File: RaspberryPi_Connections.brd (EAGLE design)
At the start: 124.4 x 101.3 mm, 4 parts

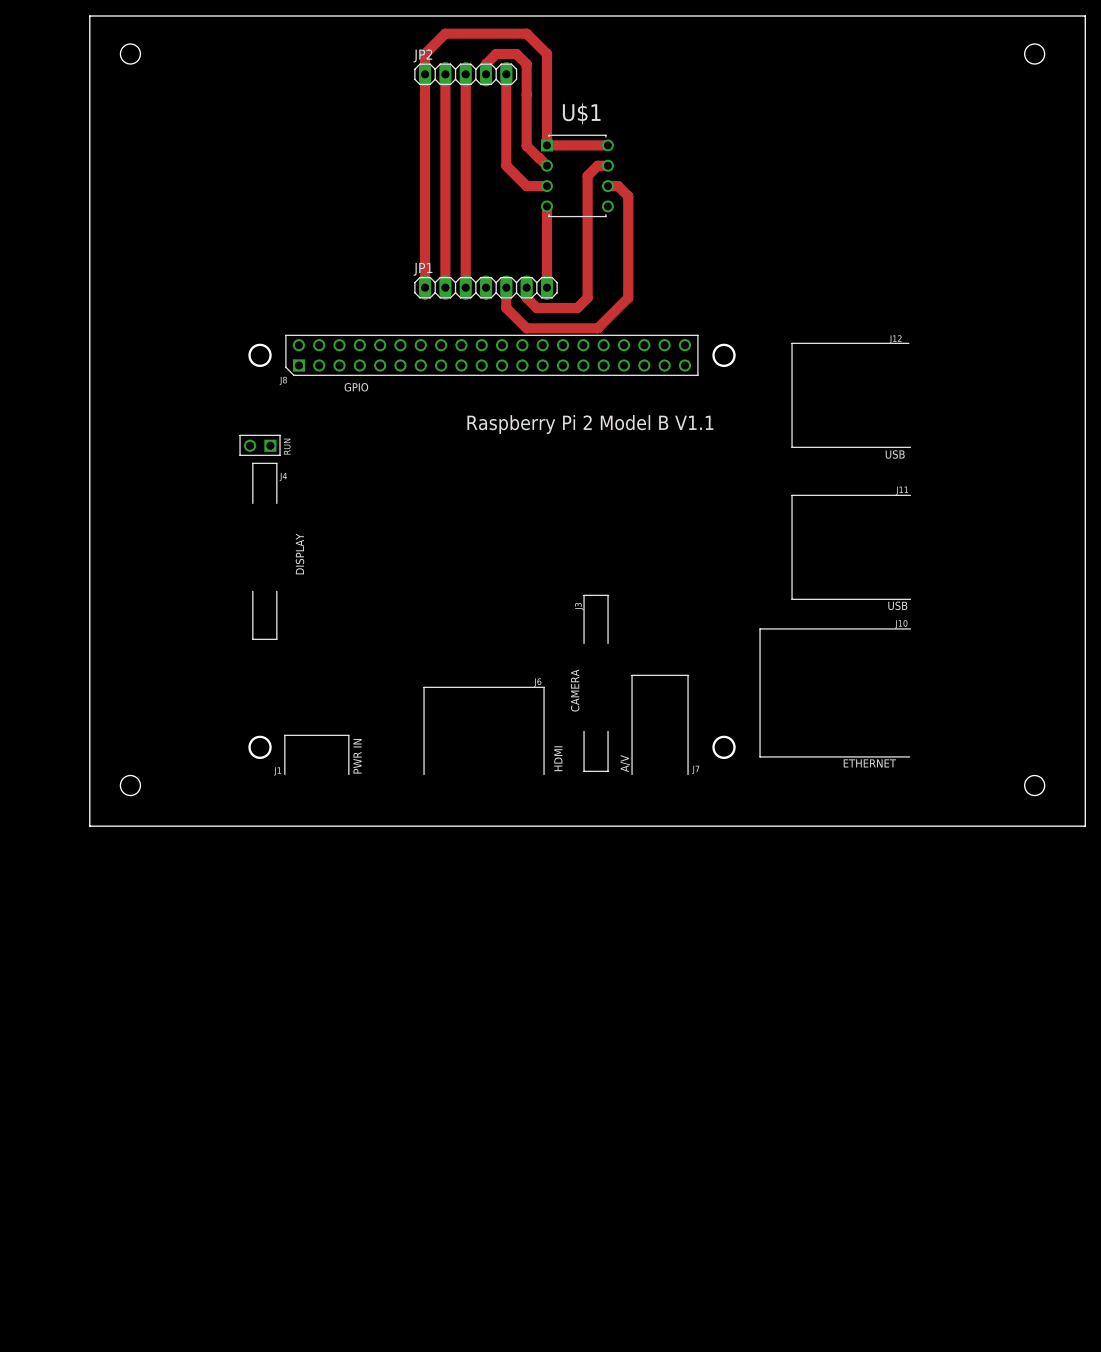
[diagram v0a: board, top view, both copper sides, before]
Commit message: Final update before printing first prototype
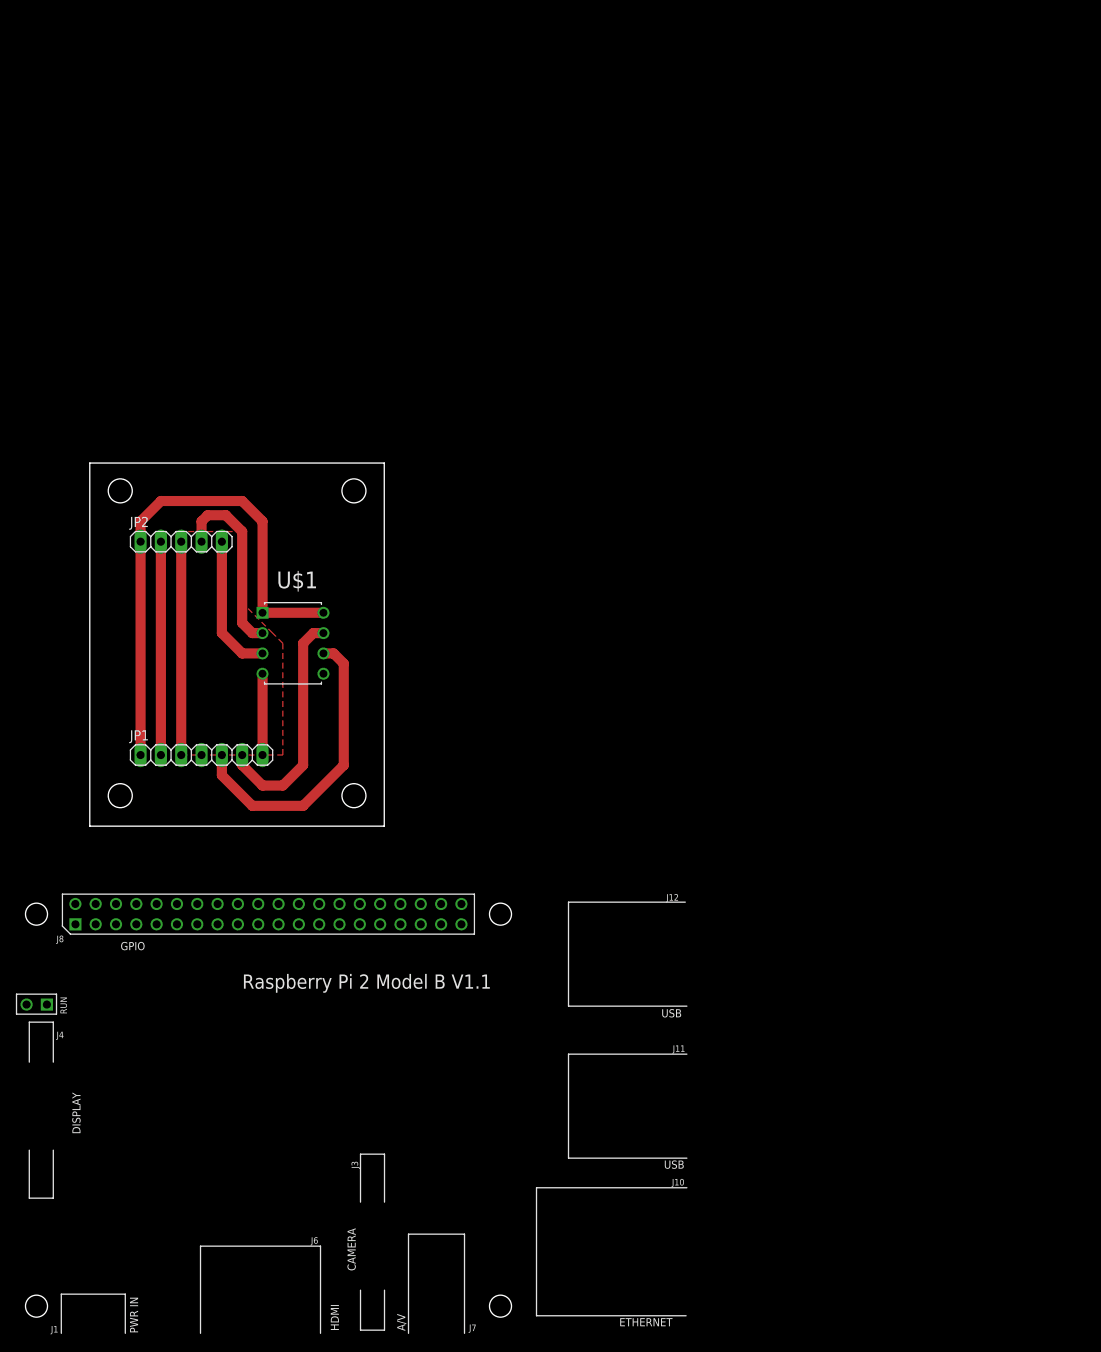
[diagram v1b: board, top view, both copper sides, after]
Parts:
- moved PCB1 75.2 mm to (-10.2, -63.5)
- moved JP1 68.4 mm to (14.0, 8.89)
- moved JP2 68.4 mm to (11.4, 35.6)
- moved U$1 68.4 mm to (29.2, 19.1)
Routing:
- net TOOL_CHANGER_ANALOG_I: track 21.2 -> 23.3 mm
- net SCLK_A: track 28.2 -> 29.3 mm
- net MISO_A: track 36.2 -> 37.2 mm
- added copper zone on layer 1, net GND_RPI
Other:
- board size 124.4 x 101.3 mm -> 36.8 x 45.4 mm
